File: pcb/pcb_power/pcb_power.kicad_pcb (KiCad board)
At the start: 2 copper layers, 100 x 79 mm, 19 parts, among them J10 JST_B4B-XH-A, J11 JST_B4P-VH, J12 XT30, K20 FINDER-40.41, K21 FINDER-40.41, Q40 BD249C, Q41 BD139, Q42 BD249C, Q43 BD139

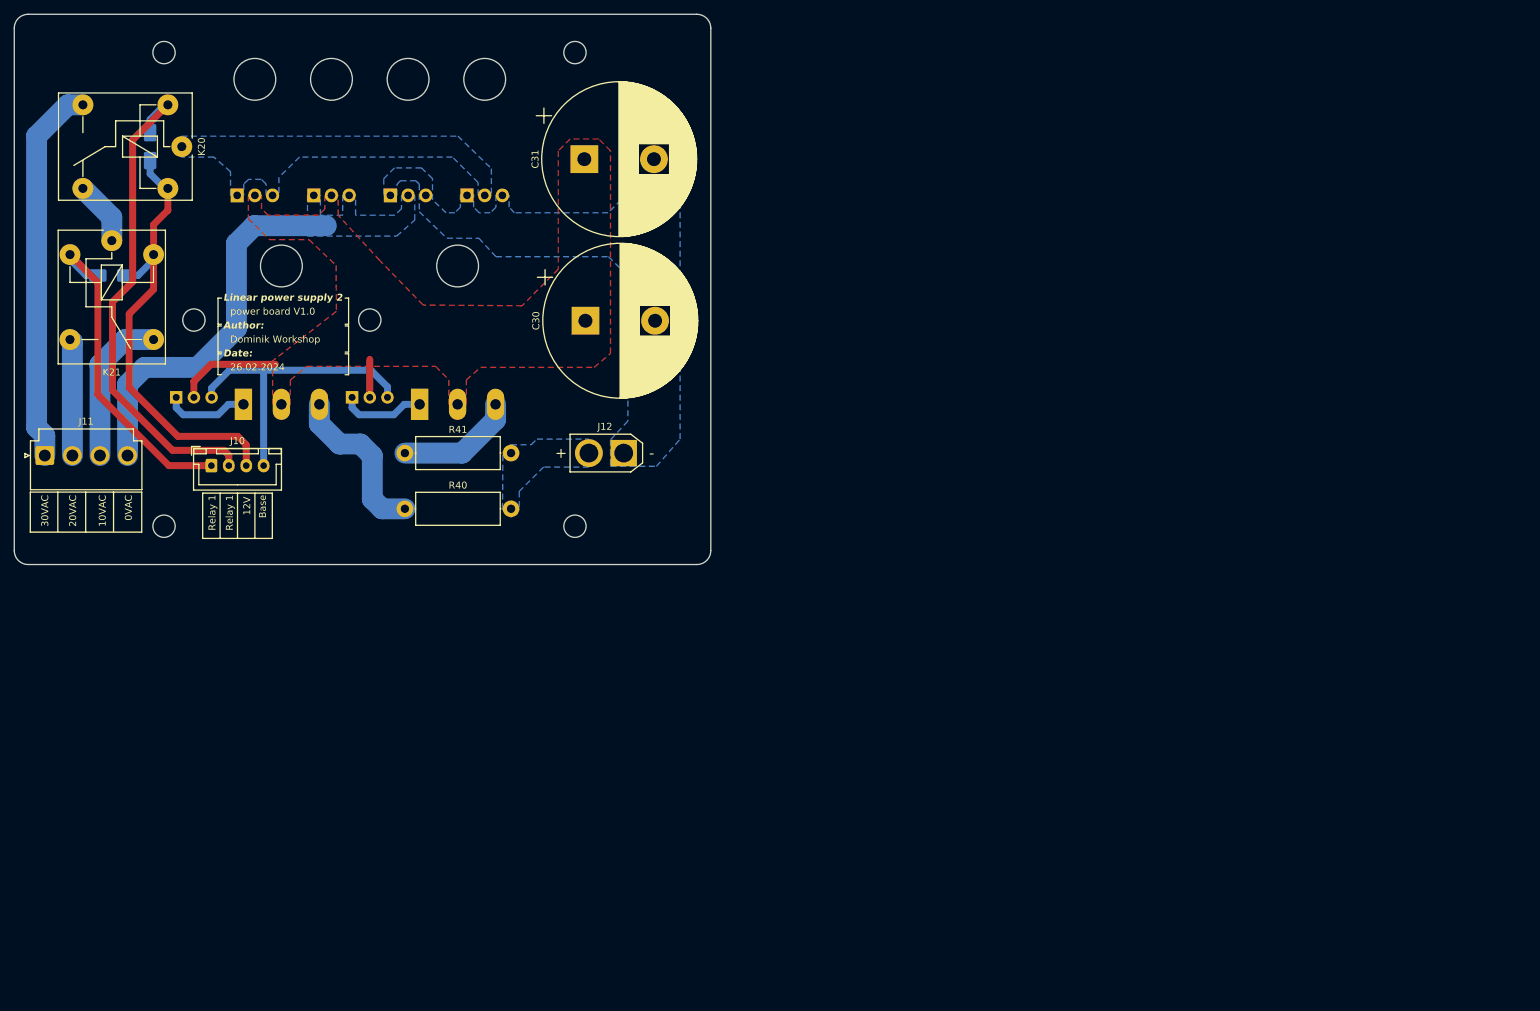
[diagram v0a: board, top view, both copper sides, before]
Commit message: centered pcb
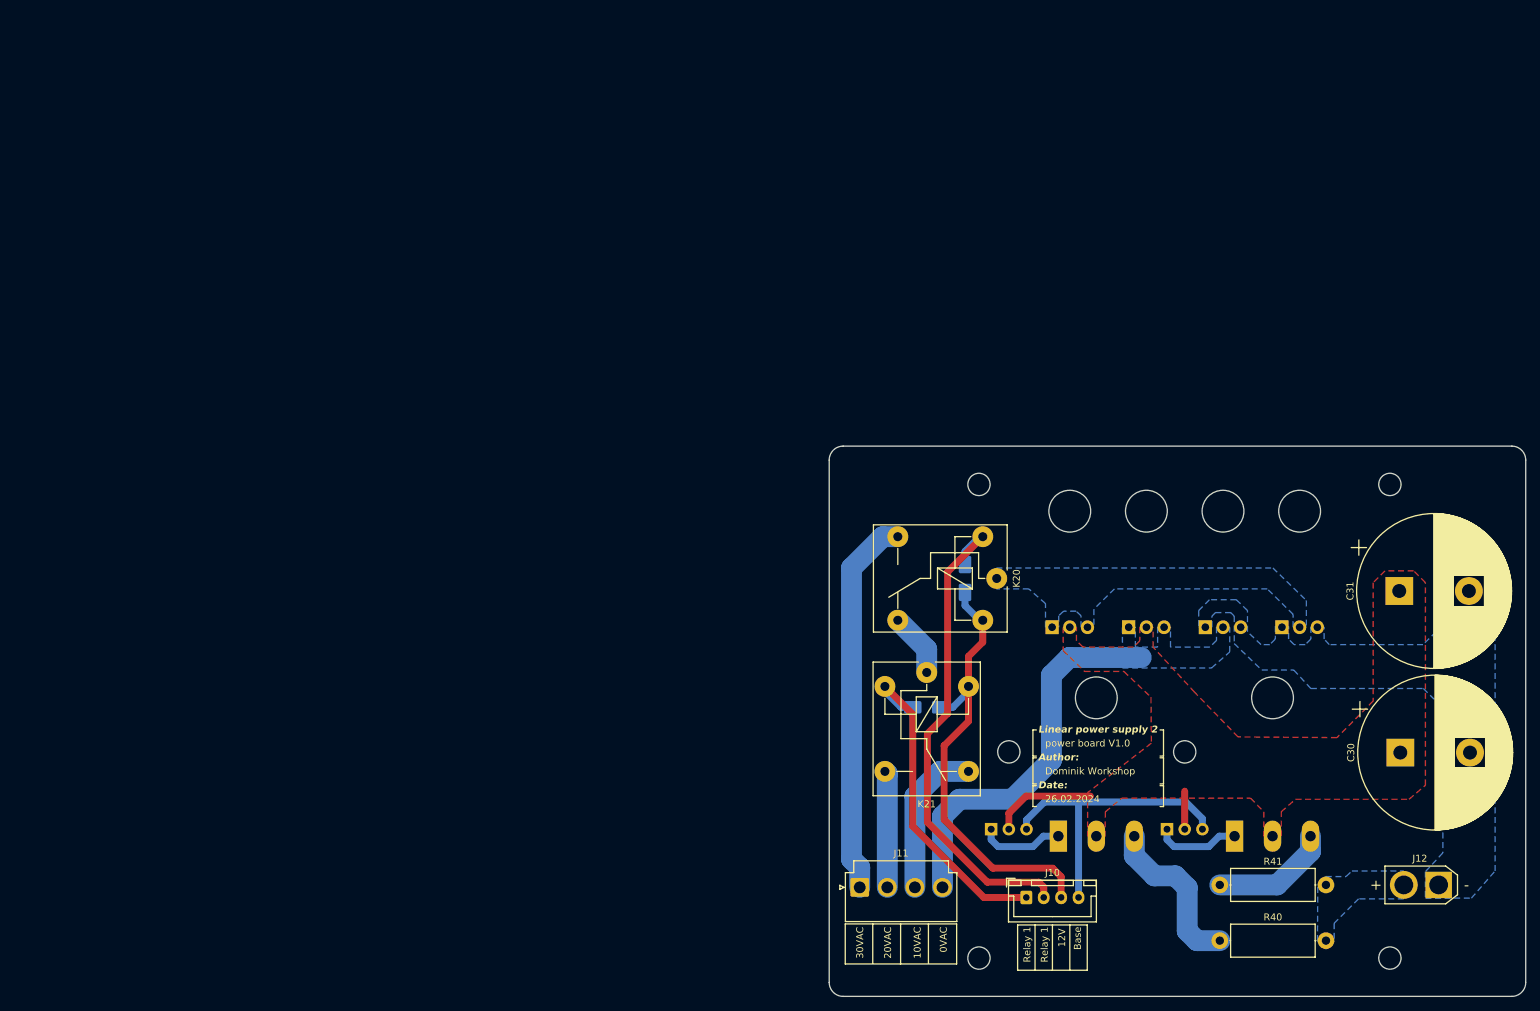
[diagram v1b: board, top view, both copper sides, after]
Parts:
- moved C31 132.4 mm to (181.8, 81.8)
- moved J10 132.4 mm to (128.3, 125.8)
- moved Q42 132.4 mm to (158.2, 117.0)
- moved R40 132.4 mm to (156.1, 132.0)
- moved R41 132.4 mm to (156.1, 124.0)
- moved C30 132.4 mm to (182.0, 105.0)
- moved D20 132.4 mm to (119.5, 80.0)
- moved D21 132.4 mm to (114.0, 98.5)
- moved D30 132.4 mm to (143.0, 87.0)
- moved D31 132.4 mm to (154.0, 87.0)
- moved D32 132.4 mm to (132.0, 87.0)
- moved D33 132.4 mm to (165.0, 87.0)
- moved J11 132.4 mm to (104.4, 124.3)
- moved J12 132.4 mm to (187.5, 124.0)
- moved K20 132.4 mm to (124.0, 80.0)
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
